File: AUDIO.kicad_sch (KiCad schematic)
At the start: 1 part, among them J8 AudioJack4

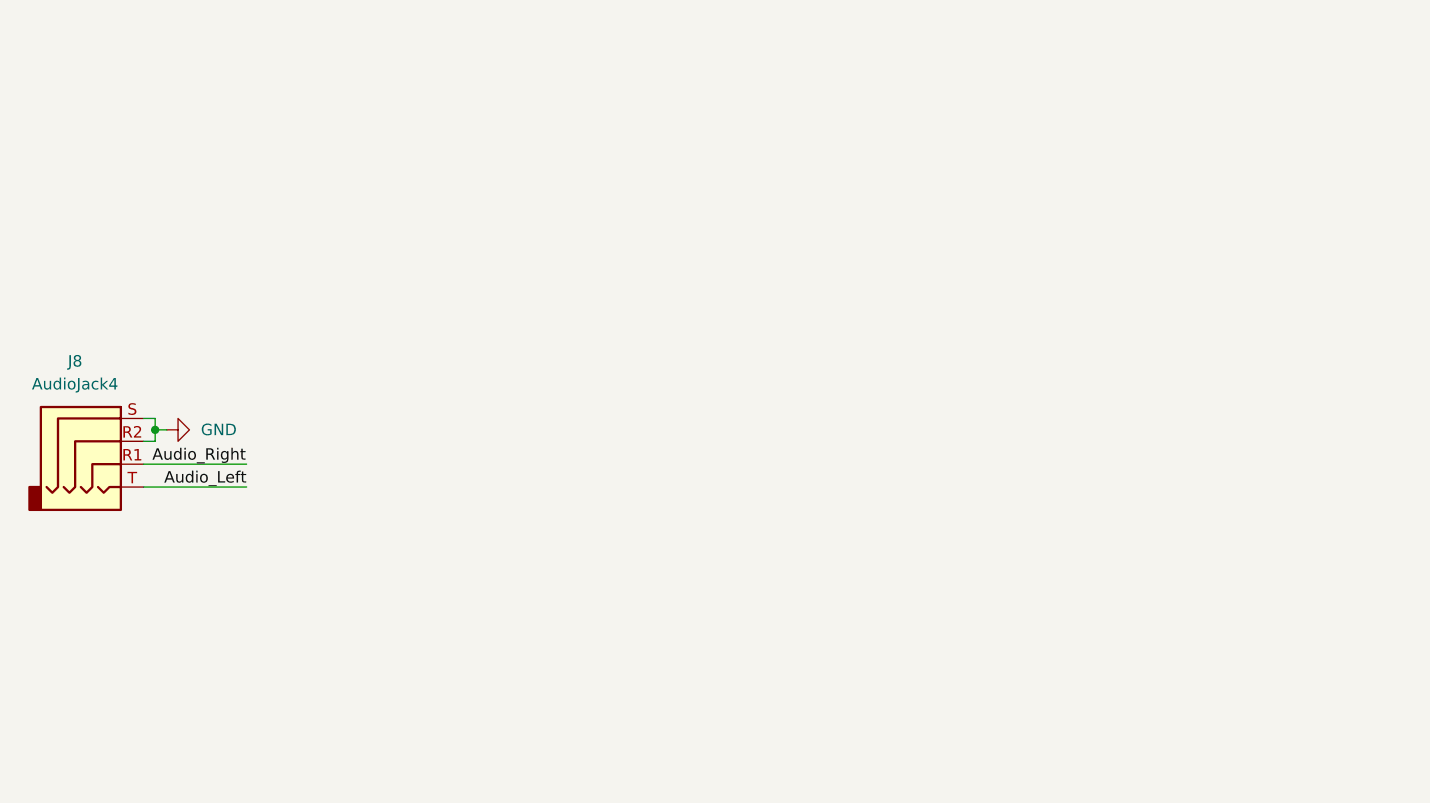
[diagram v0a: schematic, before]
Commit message: Create Audio CODEC schematic block and layout.
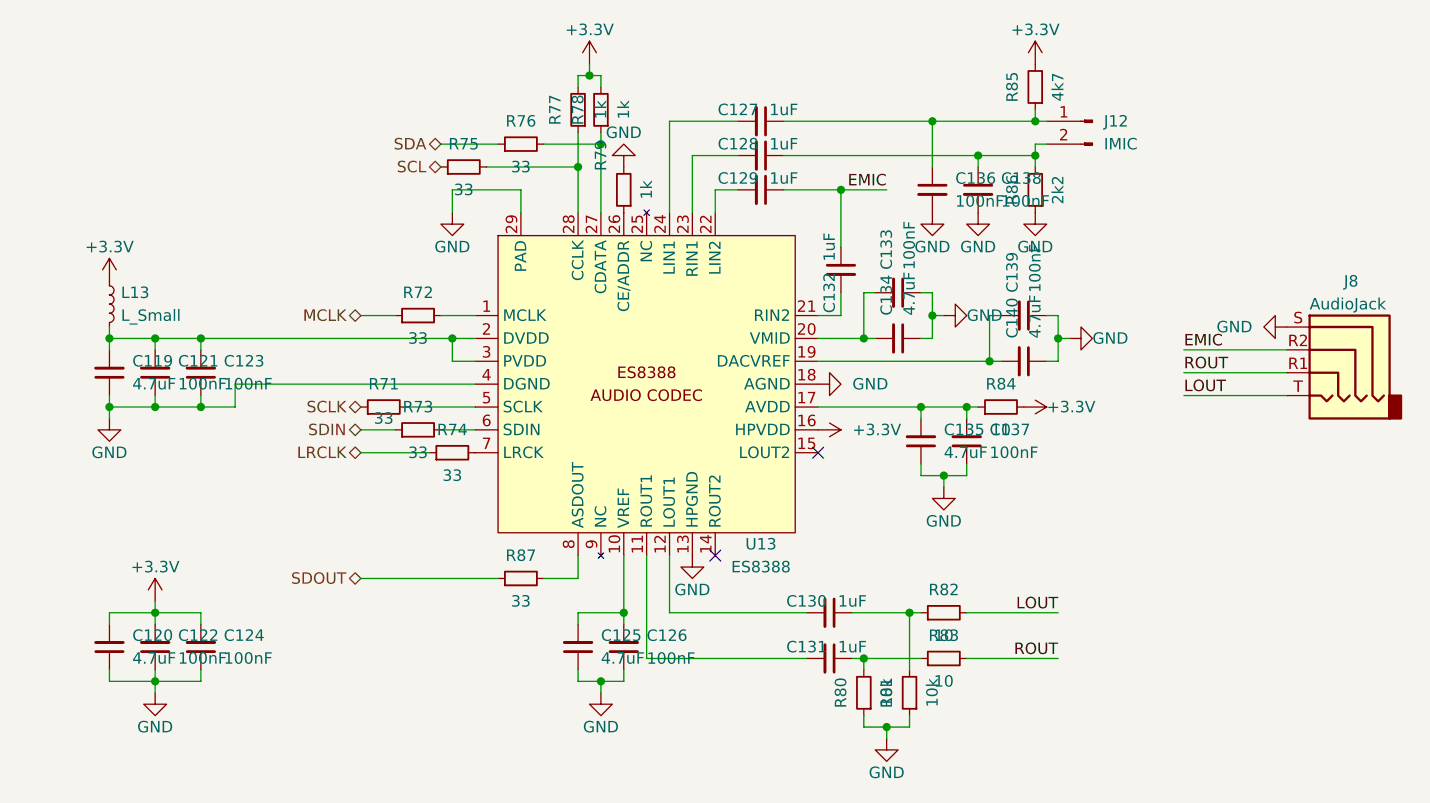
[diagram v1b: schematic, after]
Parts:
- added C119, C120, C125, C134, C135, C140: 4.7uF, Capacitor_SMD:C_0603_1608Metric, symbol Device:C_Small
- added C121, C122, C123, C124, C126, C133, C136, C137, C138, C139: 100nF, Capacitor_SMD:C_0603_1608Metric, symbol Device:C_Small
- added C127, C128, C129, C130, C131, C132: 1uF, Capacitor_SMD:C_0603_1608Metric, symbol Device:C_Small
- added J12: IMIC, Connector_PinHeader_2.54mm:PinHeader_1x02_P2.54mm_Vertical, symbol Connector:Conn_01x02_Male
- added L13: L_Small, Inductor_SMD:L_0603_1608Metric, symbol Device:L_Small
- added R71, R72, R73, R74, R75, R76, R87: 33, Resistor_SMD:R_0603_1608Metric, symbol Device:R_Small
- added R77, R78, R79: 1k, Resistor_SMD:R_0603_1608Metric, symbol Device:R_Small
- added R80, R81: 10k, Resistor_SMD:R_0603_1608Metric, symbol Device:R_Small
- added R82, R83, R84: 10, Resistor_SMD:R_0603_1608Metric, symbol Device:R_Small
- added R85: 4k7, Resistor_SMD:R_0603_1608Metric, symbol Device:R_Small
- added R86: 2k2, Resistor_SMD:R_0603_1608Metric, symbol Device:R_Small
- added U13: ES8388, Package_DFN_QFN:QFN-28-1EP_4x4mm_P0.45mm_EP2.4x2.4mm, symbol Anh_Symbols:ES8388
- J8: value AudioJack4 -> AudioJack
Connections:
- net GND: now also C119.1, C120.1, C121.1, C122.1, C123.1, C124.1, C125.1, C126.1, C133.1, C134.1, C135.1, C136.2, C137.1, C138.2, C139.1, C140.1, R79.2, R80.1, R81.1, R86.1, U13.13 (HPGND), U13.18 (AGND), U13.29 (PAD), U13.4 (DGND); no longer J8.R2
- net Audio_Left renamed LOUT
- net LOUT: now also R82.2
- net Audio_Right renamed ROUT
- net ROUT: now also R83.2
- new net: C128.1, C138.1, J12.2 (Pin_2), R86.2
- new net: C125.2, C126.2, U13.10 (VREF)
- new net: C130.1, R81.2, R82.1
- new net: R75.2, R77.1, U13.28 (CCLK)
- new net: R76.2, R78.1, U13.27 (CDATA)
- new net: R72.2, U13.1 (MCLK)
- new net: C129.2, U13.22 (LIN2)
- new net: C127.1, C136.1, J12.1 (Pin_1), R85.1
- new net: C133.2, C134.2, U13.20 (VMID)
- new net: C119.2, C121.2, C123.2, L13.2, U13.2 (DVDD), U13.3 (PVDD)
- new net: R74.2, U13.7 (LRCK)
- new net: C131.1, R80.2, R83.1
- new net: C128.2, U13.23 (RIN1)
- new net: C135.2, C137.2, R84.1, U13.17 (AVDD)
- new net: R79.1, U13.26 (CE/ADDR)
- new net: C127.2, U13.24 (LIN1)
- new net: R71.2, U13.5 (SCLK)
- new net: C132.2, U13.21 (RIN2)
- new net: C131.2, U13.11 (ROUT1)
- new net: C130.2, U13.12 (LOUT1)
- new net: C139.2, C140.2, U13.19 (DACVREF)
- new net: R73.2, U13.6 (SDIN)
- new net: R87.2, U13.8 (ASDOUT)
- new net +3.3V: C120.2, C122.2, C124.2, L13.1, R77.2, R78.2, R84.2, R85.2, U13.16 (HPVDD)
- new net EMIC: C129.1, C132.1, J8.R2
- new net LRCLK: R74.1
- new net MCLK: R72.1
- new net SCL: R75.1
- new net SCLK: R71.1
- new net SDA: R76.1
- new net SDIN: R73.1
- new net SDOUT: R87.1
- no-connect marks 0 -> 2
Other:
- moved on the sheet: J8
